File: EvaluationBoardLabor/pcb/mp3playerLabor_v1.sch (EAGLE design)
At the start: 38 parts, among them IC1 4050N, Q1 12MHz, X1 SD-Card holder, X2 1503_09

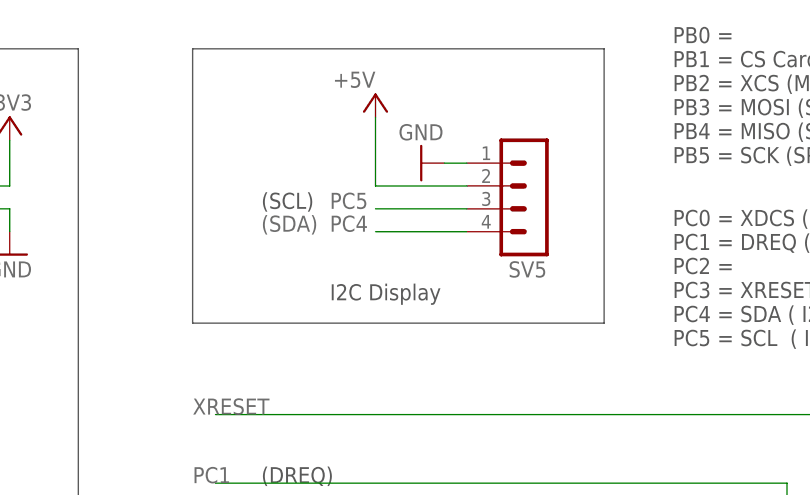
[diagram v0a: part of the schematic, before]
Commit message: update pcb
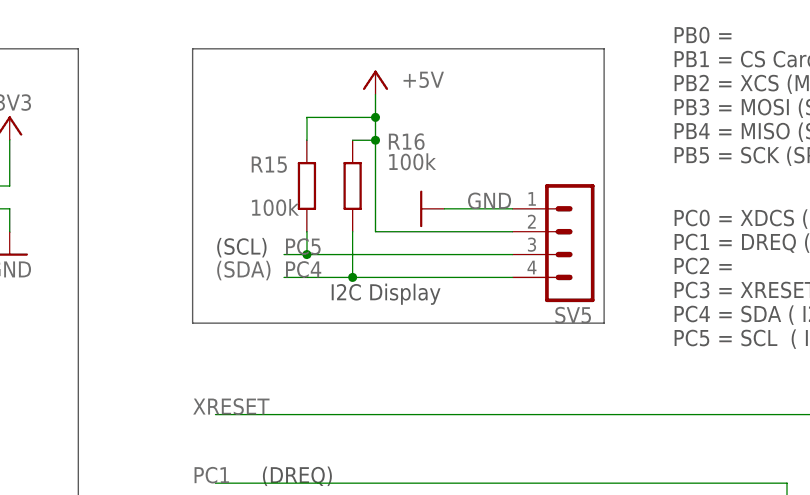
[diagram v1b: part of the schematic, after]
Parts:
- added R15, R16: 100k, rcl:R-EU_R1206
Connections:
- net +5V: now also R15.1, R16.1
- net PC4: now also R16.2
- net PC5: now also R15.2
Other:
- moved on the sheet: SV5
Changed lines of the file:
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@@
 <part name="P+6" library="supply1" library_urn="urn:adsk.eagle:library:371" deviceset="+5V" device=""/>
 <part name="P+7" library="supply1" library_urn="urn:adsk.eagle:library:371" deviceset="+5V" device=""/>
+<part name="R15" library="rcl" library_urn="urn:adsk.eagle:library:334" deviceset="R-EU_" device="R1206" package3d_urn="urn:adsk.eagle:package:23540/2" value="100k"/>
+<part name="R16" library="rcl" library_urn="urn:adsk.eagle:library:334" deviceset="R-EU_" device="R1206" package3d_urn="urn:adsk.eagle:package:23540/2" value="100k"/>
 </parts>
 <sheets>
@@
 <text x="162.56" y="76.2" size="1.778" layer="96">MP3-Decoder</text>
 <text x="96.52" y="121.92" size="1.778" layer="97">(DREQ)</text>
-<text x="96.52" y="152.4" size="1.778" layer="97">(SCL)</text>
-<text x="96.52" y="149.86" size="1.778" layer="96">(SDA)</text>
+<text x="91.44" y="147.32" size="1.778" layer="97">(SCL)</text>
+<text x="91.44" y="144.78" size="1.778" layer="96">(SDA)</text>
 <wire x1="88.9" y1="170.18" x2="134.62" y2="170.18" width="0.1524" layer="97"/>
 <wire x1="134.62" y1="170.18" x2="134.62" y2="139.7" width="0.1524" layer="97"/>
@@
 <attribute name="VALUE" x="71.12" y="165.1" size="1.778" layer="96" rot="R180"/>
 </instance>
-<instance part="SV5" gate="1" x="127" y="152.4" smashed="yes" rot="R180">
-<attribute name="VALUE" x="128.27" y="162.56" size="1.778" layer="96" rot="R180"/>
-<attribute name="NAME" x="128.27" y="146.558" size="1.778" layer="95" rot="R180"/>
-</instance>
-<instance part="GND16" gate="1" x="114.3" y="157.48" smashed="yes" rot="R270">
-<attribute name="VALUE" x="111.76" y="160.02" size="1.778" layer="96"/>
-</instance>
-<instance part="P+2" gate="1" x="109.22" y="165.1" smashed="yes">
-<attribute name="VALUE" x="109.22" y="167.64" size="1.778" layer="96" rot="R180"/>
+<instance part="SV5" gate="1" x="132.08" y="147.32" smashed="yes" rot="R180">
+<attribute name="VALUE" x="133.35" y="157.48" size="1.778" layer="96" rot="R180"/>
+<attribute name="NAME" x="133.35" y="141.478" size="1.778" layer="95" rot="R180"/>
+</instance>
+<instance part="GND16" gate="1" x="114.3" y="152.4" smashed="yes" rot="R270">
+<attribute name="VALUE" x="119.38" y="152.4" size="1.778" layer="96"/>
+</instance>
+<instance part="P+2" gate="1" x="109.22" y="167.64" smashed="yes">
+<attribute name="VALUE" x="116.84" y="167.64" size="1.778" layer="96" rot="R180"/>
 </instance>
 <instance part="R2" gate="G$1" x="226.06" y="144.78" smashed="yes" rot="R270">
@@
 <instance part="P+7" gate="1" x="185.42" y="53.34" smashed="yes">
 <attribute name="VALUE" x="185.42" y="55.88" size="1.778" layer="96" rot="R180"/>
+</instance>
+<instance part="R15" gate="G$1" x="101.6" y="154.94" smashed="yes" rot="R270">
+<attribute name="NAME" x="95.25" y="156.4386" size="1.778" layer="95"/>
+<attribute name="VALUE" x="95.25" y="151.638" size="1.778" layer="96"/>
+</instance>
+<instance part="R16" gate="G$1" x="106.68" y="154.94" smashed="yes" rot="R270">
+<attribute name="NAME" x="110.49" y="158.9786" size="1.778" layer="95"/>
+<attribute name="VALUE" x="110.49" y="156.718" size="1.778" layer="96"/>
 </instance>
 </instances>
@@
 <pinref part="SV5" gate="1" pin="1"/>
 <pinref part="GND16" gate="1" pin="GND"/>
-<wire x1="119.38" y1="157.48" x2="116.84" y2="157.48" width="0.1524" layer="91"/>
+<wire x1="124.46" y1="152.4" x2="116.84" y2="152.4" width="0.1524" layer="91"/>
 </segment>
 <segment>
@@
 <pinref part="SV5" gate="1" pin="2"/>
 <pinref part="P+2" gate="1" pin="+5V"/>
-<wire x1="119.38" y1="154.94" x2="109.22" y2="154.94" width="0.1524" layer="91"/>
-<wire x1="109.22" y1="154.94" x2="109.22" y2="162.56" width="0.1524" layer="91"/>
+<wire x1="124.46" y1="149.86" x2="109.22" y2="149.86" width="0.1524" layer="91"/>
+<wire x1="109.22" y1="149.86" x2="109.22" y2="160.02" width="0.1524" layer="91"/>
+<pinref part="R16" gate="G$1" pin="1"/>
+<wire x1="109.22" y1="160.02" x2="109.22" y2="162.56" width="0.1524" layer="91"/>
+<wire x1="109.22" y1="162.56" x2="109.22" y2="165.1" width="0.1524" layer="91"/>
+<wire x1="106.68" y1="160.02" x2="109.22" y2="160.02" width="0.1524" layer="91"/>
+<junction x="109.22" y="160.02"/>
+<pinref part="R15" gate="G$1" pin="1"/>
+<wire x1="101.6" y1="160.02" x2="101.6" y2="162.56" width="0.1524" layer="91"/>
+<wire x1="101.6" y1="162.56" x2="109.22" y2="162.56" width="0.1524" layer="91"/>
+<junction x="109.22" y="162.56"/>
 </segment>
 <segment>
@@
 <segment>
 <pinref part="SV5" gate="1" pin="4"/>
-<wire x1="119.38" y1="149.86" x2="109.22" y2="149.86" width="0.1524" layer="91"/>
-<label x="104.14" y="149.86" size="1.778" layer="95"/>
+<wire x1="124.46" y1="144.78" x2="106.68" y2="144.78" width="0.1524" layer="91"/>
+<label x="99.06" y="144.78" size="1.778" layer="95"/>
+<pinref part="R16" gate="G$1" pin="2"/>
+<wire x1="106.68" y1="144.78" x2="99.06" y2="144.78" width="0.1524" layer="91"/>
+<wire x1="106.68" y1="149.86" x2="106.68" y2="144.78" width="0.1524" layer="91"/>
+<junction x="106.68" y="144.78"/>
 </segment>
 </net>
@@
 <segment>
 <pinref part="SV5" gate="1" pin="3"/>
-<wire x1="119.38" y1="152.4" x2="109.22" y2="152.4" width="0.1524" layer="91"/>
-<label x="104.14" y="152.4" size="1.778" layer="95"/>
-</segment>
-</net>
+<wire x1="124.46" y1="147.32" x2="101.6" y2="147.32" width="0.1524" layer="91"/>
+<label x="99.06" y="147.32" size="1.778" layer="95"/>
+<pinref part="R15" gate="G$1" pin="2"/>
+<wire x1="101.6" y1="147.32" x2="99.06" y2="147.32" width="0.1524" layer="91"/>
+<wire x1="101.6" y1="149.86" x2="101.6" y2="147.32" width="0.1524" layer="91"/>
+<junction x="101.6" y="147.32"/>
+</segment>
+</net>
